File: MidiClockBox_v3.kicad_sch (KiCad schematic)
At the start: 58 parts, among them J1 Midi In 0, J10 Display, J11 Midi Out 3, J12 Midi Out 4, J13 Midi Out 5, J14 Sync Out 0, J15 Sync Out 1, J2 ICSP, J3 Conn_02x09_Odd_Even, J4 Conn_02x04_Odd_Even, J5 Conn_02x12_Counter_Clockwise, J6 Midi Out 0, J7 Midi Out 1, J8 Midi Out 2, J9 WS2812, SW1 RotaryEncoder_Switch, U1 CD74HC4067SM, U2 74LS241, U3 6N138

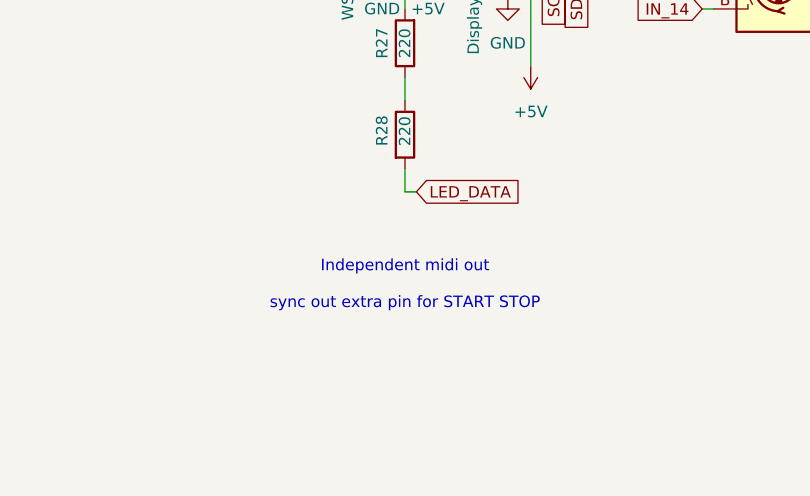
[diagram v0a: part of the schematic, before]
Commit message: add comments for stuff 2do
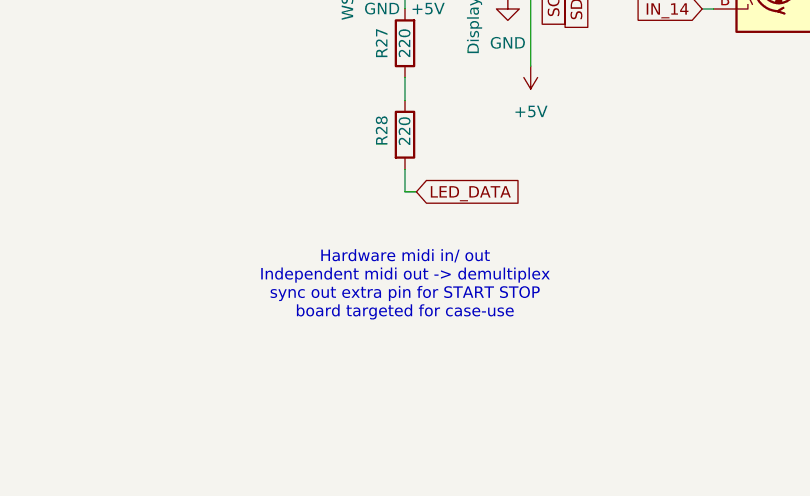
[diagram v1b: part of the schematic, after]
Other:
- note added: "Hardware midi in/ out Independent midi out -> demultiplex sync out extra pin for START STOP board targeted for case-use"
- note removed: "Independent midi out sync out extra pin for START STOP"
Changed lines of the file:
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@@
 		)
 	)
-	(text "Independent midi out\n\nsync out extra pin for START STOP"
+	(text "Hardware midi in/ out\nIndependent midi out -> demultiplex\nsync out extra pin for START STOP\nboard targeted for case-use\n"
 		(exclude_from_sim no)
 		(at 227.33 172.974 0)

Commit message: add stuff
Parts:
- added C3, C4, C5, C6, C7: 0.1µ, Capacitor_SMD:C_0603_1608Metric, symbol Device:C
- added J16: Conn_01x08, Connector_PinHeader_2.54mm:PinHeader_1x08_P2.54mm_Vertical, symbol Connector_Generic:Conn_01x08
- added U4: 74HC595, Package_SO:TSSOP-28_6.1x9.7mm_P0.65mm, symbol 74xx:74HC595
- added U6, U7: 74LS08, symbol 74xx:74LS08
- added U8: 74HC595, symbol 74xx:74HC595
- added U9: 74LS241, Package_SO:SOIC-20W_7.5x12.8mm_P1.27mm, symbol 74xx:74LS241
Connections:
- net +5V: now also C3.1, C4.1, C5.1, C6.1, C7.1, J16.7 (Pin_7), U4.10 (~{SRCLR}), U4.16 (VCC), U6.14 (VCC), U7.14 (VCC), U8.10 (~{SRCLR}), U8.16 (VCC), U9.19 (OEb), U9.20 (VCC)
- net GND: now also C3.2, C4.2, C5.2, C6.2, C7.2, J16.8 (Pin_8), U4.13 (~{OE}), U4.8 (GND), U6.7 (GND), U7.7 (GND), U8.13 (~{OE}), U8.8 (GND), U9.1 (OEa), U9.10 (GND)
- net MIDI_TX: now also U6.1, U6.12, U6.4, U6.9, U7.1, U7.9; no longer U2.11 (I0b), U2.13 (I1b), U2.2 (I0a), U2.4 (I1a), U2.6 (I2a), U2.8 (I3a)
- net SYNC_TX: now also U7.12, U7.4; no longer U2.15 (I2b), U2.17 (I3b)
- net SYNC_START_STOP_BUFFERED_1: now reaches J15.R
- net SYNC_START_STOP_BUFFERED_1: now also U9.16 (O1a)
- net DA2: now reaches J5.18 (Pin_18)
- net DA2: now also U4.12 (RCLK), U8.12 (RCLK)
- net SYNC_START_STOP: now reaches J5.20 (Pin_20)
- net SYNC_START_STOP: now also U9.2 (I0a), U9.4 (I1a)
- net DA0: now reaches J5.7 (Pin_7)
- net DA0: now also U8.14 (SER)
- net DA1: now reaches J5.8 (Pin_8)
- net DA1: now also U4.11 (SRCLK), U8.11 (SRCLK)
- net SYNC_START_STOP_BUFFERED_0: now reaches J14.R
- net SYNC_START_STOP_BUFFERED_0: now also U9.18 (O0a)
- net SYNC_OUT_0 renamed SYNC_TX_BUFFERED_0
- net SYNC_OUT_1 renamed SYNC_TX_BUFFERED_1
- new net: U2.11 (I0b), U7.3
- new net: U2.13 (I1b), U7.8
- new net: U2.15 (I2b), U7.11
- new net: U2.17 (I3b), U7.6
- new net: U2.2 (I0a), U6.3
- new net: U2.4 (I1a), U6.6
- new net: U2.6 (I2a), U6.8
- new net: U2.8 (I3a), U6.11
- new net: J16.1 (Pin_1), U9.14 (O2a)
- new net: J16.2 (Pin_2), U9.12 (O3a)
- new net: J16.3 (Pin_3), U9.9 (O0b)
- new net: J16.4 (Pin_4), U9.7 (O1b)
- new net: J16.5 (Pin_5), U9.5 (O2b)
- new net: J16.6 (Pin_6), U9.3 (O3b)
- new net: U6.2, U8.15 (QA)
- new net: U7.13, U8.6 (QG)
- new net: U4.1 (QB), U9.8 (I3a)
- new net: U4.14 (SER), U8.9 (QH')
- new net: U4.15 (QA), U9.6 (I2a)
- new net: U4.2 (QC), U9.11 (I0b)
- new net: U4.3 (QD), U9.13 (I1b)
- new net: U4.4 (QE), U9.15 (I2b)
- new net: U4.5 (QF), U9.17 (I3b)
- new net: U6.13, U8.3 (QD)
- new net: U7.5, U8.7 (QH)
- new net: U6.10, U8.2 (QC)
- new net: U6.5, U8.1 (QB)
- new net: U7.10, U8.5 (QF)
- new net: U7.2, U8.4 (QE)
- no-connect marks 8 -> 5
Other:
- note added: "D19 / A1"
- note added: "D4 / A6"
- note added: "D5"
- note added: "Hardware midi in/ out: check Independent midi out -> demultiplex: check sync out extra pin for START STOP: check board targeted for case-use Potentialfreie Kontakte"
- note added: "Pre-load MIDI and SYNC outputs"
- note added: "SYNC START STOP sind nicht unabhängig, aber es gibt 6 gepufferte Ausgänge mit VCC und GND zum Forschen"
- note removed: "Hardware midi in/ out Independent midi out -> demultiplex sync out extra pin for START STOP board targeted for case-use"
- moved on the sheet: C1, C2, D1, J1, J10, J11, J12, J13, J14, J15, J2, J3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
